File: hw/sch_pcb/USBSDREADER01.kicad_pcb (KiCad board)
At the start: 2 copper layers, 40.1 x 40.1 mm, 8 parts, among them J1 Umin ... Umax, M1 HOLE M3, M2 HOLE M3, M3 HOLE, M4 HOLE

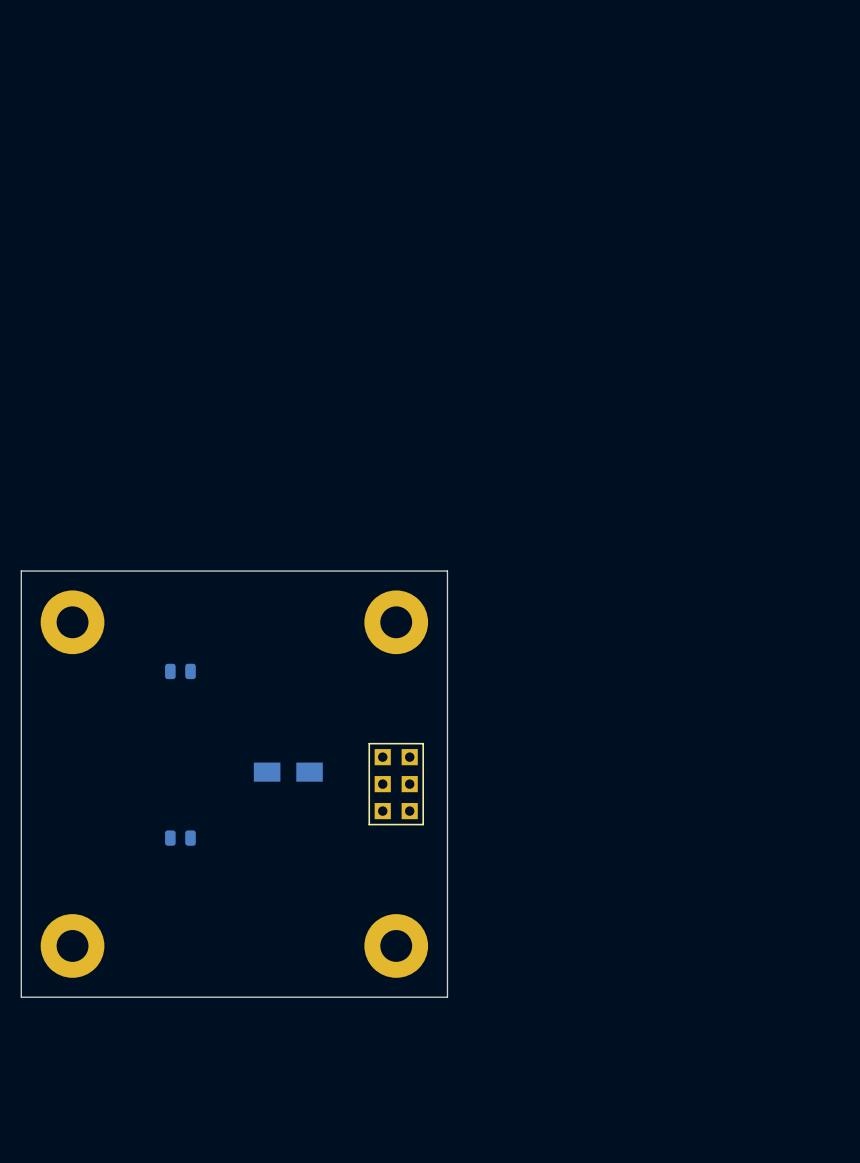
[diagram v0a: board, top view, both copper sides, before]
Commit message: wip
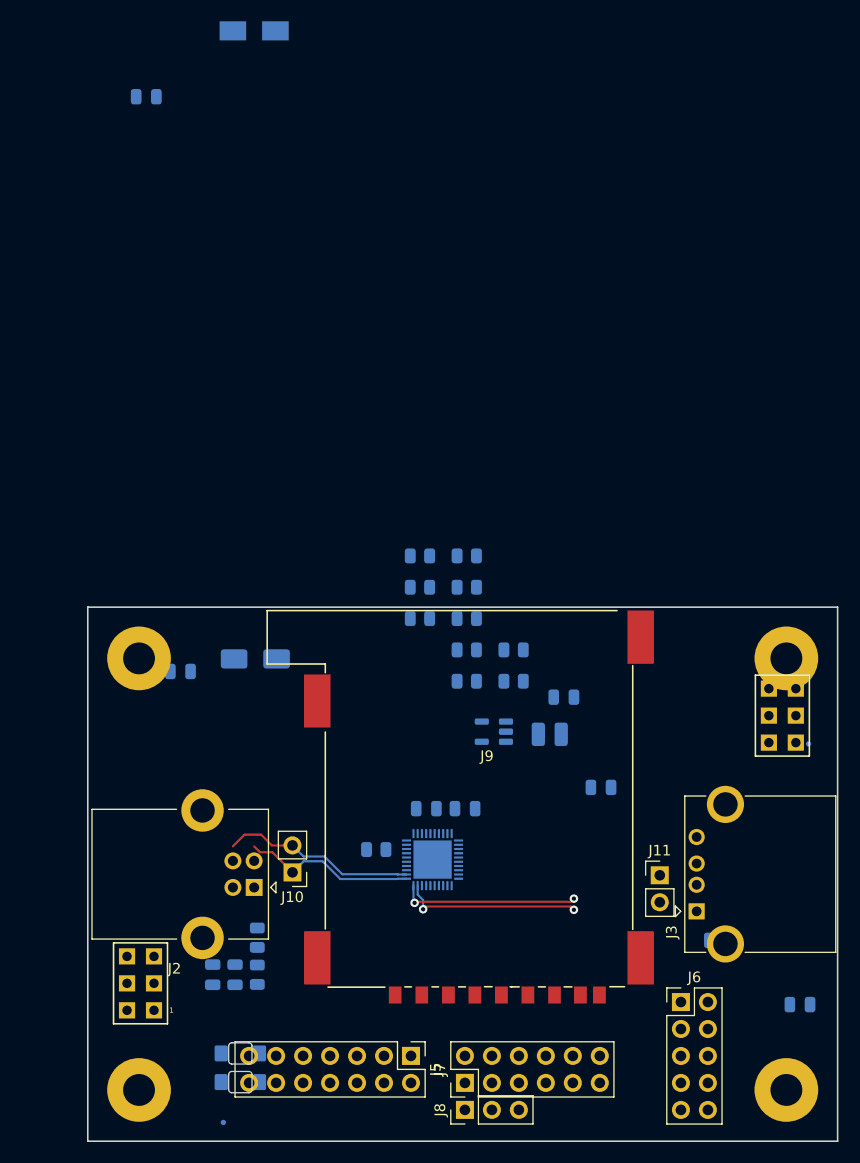
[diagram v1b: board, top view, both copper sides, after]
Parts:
- added C10: 100nF, Capacitor_SMD:C_0805_2012Metric, B.Cu at (125.0, 114.5)
- added C3: C_Small, Capacitor_SMD:C_0805_2012Metric, B.Cu at (148.7, 98.8)
- added C4: C_Small, Capacitor_SMD:C_0805_2012Metric, B.Cu at (161.5, 96.8)
- added C5: C_Small, Capacitor_SMD:C_0805_2012Metric, B.Cu at (145.1, 98.8)
- added C6: C_Small, Capacitor_SMD:C_0805_2012Metric, B.Cu at (172.7, 111.2)
- added C7: C_Small, Capacitor_SMD:C_0805_2012Metric, B.Cu at (180.3, 117.3)
- added C8: 10uF, Capacitor_SMD:C_0805_2012Metric, B.Cu at (158.0, 88.3)
- added C9: 10uF, Capacitor_SMD:C_0805_2012Metric, B.Cu at (127.1, 114.5)
- added D2: BZV55C-5,6V, Diode_SMD:D_SMA, B.Cu at (129.0, 84.7)
- added D3: LED, Mlab_D:LED_1206_mill, B.Cu at (127.6, 124.6)
- added D4: LED, Mlab_D:LED_1206_mill, B.Cu at (127.6, 121.9)
- added FID1: Fiducial, Fiducial:Fiducial_0.5mm_Mask1mm, B.Cu at (126.0, 128.4)
- added FID2: Fiducial, Fiducial:Fiducial_0.5mm_Mask1mm, B.Cu at (181.1, 92.7)
- added IC1: MAX14502AETL+, Mlab_IO:QFN40P500X500X80-41N, B.Cu at (145.7, 103.6)
- added J10: HEADER_1x02, Connector_PinHeader_2.54mm:PinHeader_1x02_P2.54mm_Vertical, F.Cu at (132.5, 104.8)
- added J11: HEADER_1x02, Connector_PinHeader_2.54mm:PinHeader_1x02_P2.54mm_Vertical, F.Cu at (167.1, 105.1)
- added J2: USB_B, Connector_USB:USB_B_Lumberg_2411_02_Horizontal, F.Cu at (128.9, 106.2)
- added J3: USB_A, Connector_USB:USB_A_CONNFLY_DS1095-WNR0, F.Cu at (170.5, 108.5)
- added J4: VBUS, Mlab_Pin_Headers:Straight_2x03, F.Cu at (118.2, 115.3)
- added J5: HEADER_2x07_PARALLEL, Connector_PinHeader_2.54mm:PinHeader_2x07_P2.54mm_Vertical, F.Cu at (143.6, 122.1)
- added J6: HEADER_2x05_PARALLEL, Connector_PinHeader_2.54mm:PinHeader_2x05_P2.54mm_Vertical, F.Cu at (169.1, 117.0)
- added J7: HEADER_2x04_PARALLEL, Connector_PinHeader_2.54mm:PinHeader_2x06_P2.54mm_Vertical, F.Cu at (148.7, 124.7)
- added J8: HEADER_1x02, Connector_PinHeader_2.54mm:PinHeader_1x03_P2.54mm_Vertical, F.Cu at (148.7, 127.2)
- added J9: SD_Card-FPS009-4200-0, Mlab_CON:FPS009-4200-0, F.Cu at (150.0, 80.2)
- added L1: 1uH, Inductor_SMD:L_1008_2520Metric, B.Cu at (156.7, 91.8)
- added R1: 6.19k, Resistor_SMD:R_0805_2012Metric, B.Cu at (140.4, 102.7)
- added R10: R_Small, Resistor_SMD:R_0805_2012Metric, B.Cu at (148.9, 86.8)
- added R11: R_Small, Resistor_SMD:R_0805_2012Metric, B.Cu at (144.5, 75.0)
- added R12: 10k, Resistor_SMD:R_0805_2012Metric, B.Cu at (144.5, 78.0)
- added R13: 10k, Resistor_SMD:R_0805_2012Metric, B.Cu at (144.5, 80.9)
- added R2: 10k, Resistor_SMD:R_0805_2012Metric, B.Cu at (129.2, 114.5)
- added R3: 10k, Resistor_SMD:R_0805_2012Metric, B.Cu at (129.2, 111.0)
- added R4: 10k, Resistor_SMD:R_0805_2012Metric, B.Cu at (153.3, 83.9)
- added R5: 10k, Resistor_SMD:R_0805_2012Metric, B.Cu at (153.3, 86.8)
- added R6: R_Small, Resistor_SMD:R_0805_2012Metric, B.Cu at (148.9, 75.0)
- added R7: R_Small, Resistor_SMD:R_0805_2012Metric, B.Cu at (148.9, 78.0)
- added R8: R_Small, Resistor_SMD:R_0805_2012Metric, B.Cu at (148.9, 80.9)
- added R9: R_Small, Resistor_SMD:R_0805_2012Metric, B.Cu at (148.9, 83.9)
- added U1: TS5A4594, Package_TO_SOT_SMD:SOT-23-5, B.Cu at (151.4, 91.6)
- J1: value Umin ... Umax -> 3.3V
- moved C1 69.9 mm to (118.7, 31.8)
- moved D1 69.9 mm to (128.9, 25.6)
- moved M2 67.3 mm to (179.0, 84.7)
- moved M4 39.2 mm to (179.0, 125.3)
- moved J1 36.9 mm to (178.6, 90.1), turned to 0 degrees
- moved M1 24.5 mm to (118.0, 84.7)
- moved M3 14.9 mm to (118.0, 125.3)
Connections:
- net +5V renamed VCC
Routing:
- net /USB_IN_D+: track 0.00 -> 18.4 mm
- net /USB_OUT_D-: track 0.00 -> 16.9 mm, vias 0 -> 2
- net /USB_OUT_D+: track 0.00 -> 16.8 mm, vias 0 -> 2
- net /USB_IN_D-: track 0.00 -> 16.5 mm
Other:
- board size 40.1 x 40.1 mm -> 70.6 x 50.3 mm
